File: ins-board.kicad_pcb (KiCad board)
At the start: 2 copper layers, 35 x 20 mm, 48 parts, among them P1 CONN_8, P2 PWR, U1 STM32F042C6T6, U2 MIC5201-3.3YS, U3 H3LIS331DL, U4 MPU6000, U5 LPS331AP, X1 CRYSTAL 16MHz 10ppm

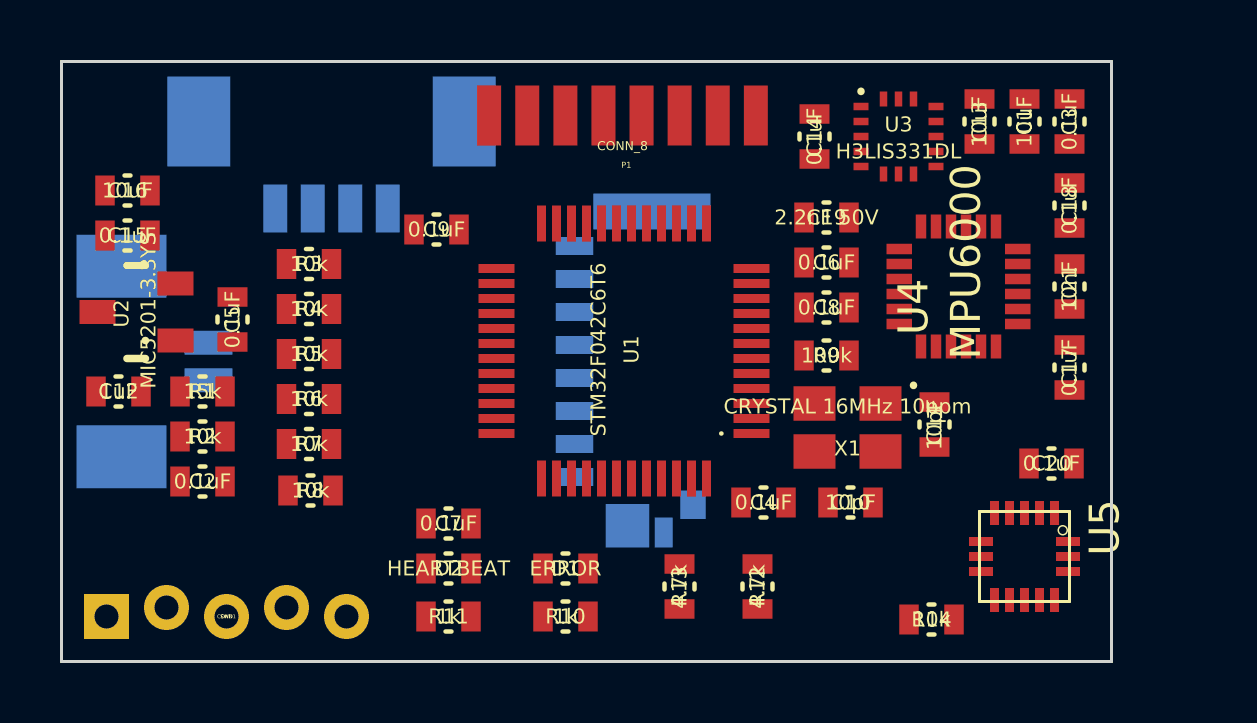
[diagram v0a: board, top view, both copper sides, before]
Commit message: Routing
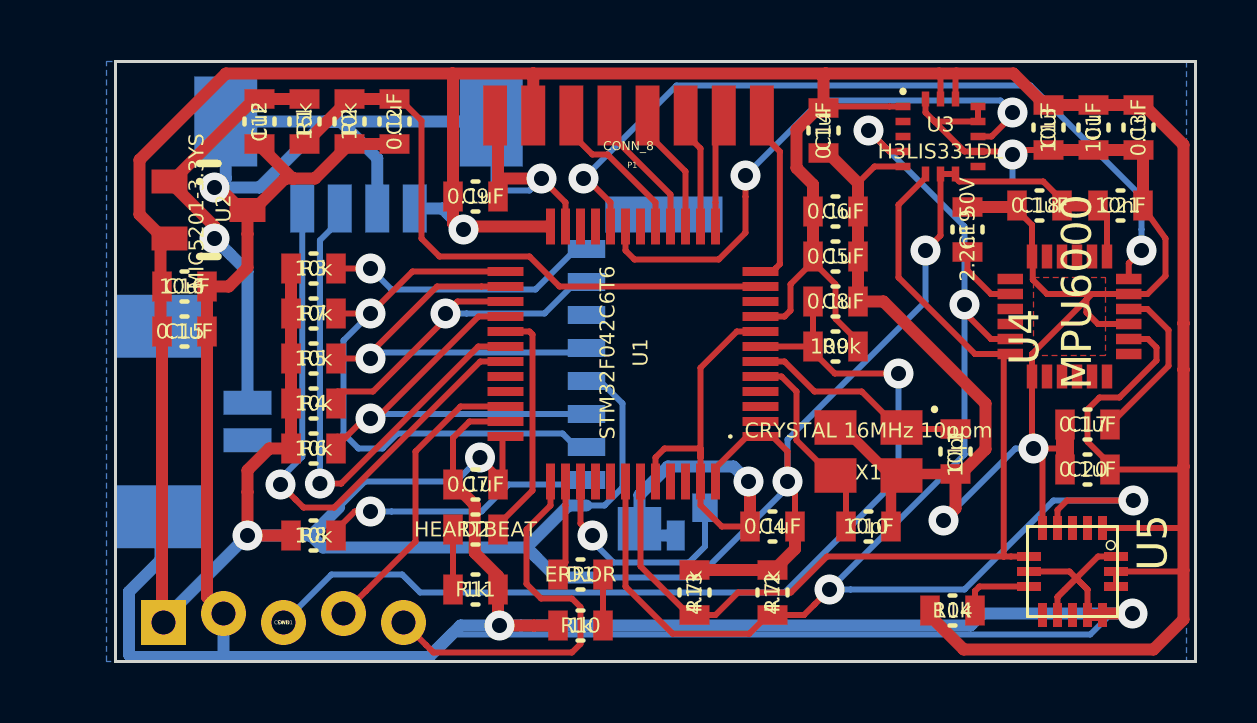
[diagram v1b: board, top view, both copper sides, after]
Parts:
- moved C5 20.2 mm to (158.8, 94.0), turned to 0 degrees
- moved C2 13.6 mm to (144.1, 89.5), turned to 270 degrees
- moved R2 11.6 mm to (142.6, 89.5), turned to 270 degrees
- moved C12 10.2 mm to (139.6, 89.5), turned to 270 degrees
- moved R1 9.62 mm to (141.1, 89.5), turned to 90 degrees
- moved U2 5.30 mm to (136.6, 91.5), turned to 270 degrees
- moved C19 4.72 mm to (163.2, 93.1), turned to 90 degrees
- moved R7 4.35 mm to (141.4, 95.9)
- moved U4 3.83 mm to (166.6, 96.0)
- moved C15 3.72 mm to (137.1, 96.5), turned to 0 degrees
- moved C16 3.72 mm to (137.1, 95.0), turned to 0 degrees
- moved C21 3.19 mm to (168.3, 92.3), turned to 0 degrees
- moved R4 3.15 mm to (141.4, 98.9)
- moved P2 2.39 mm to (136.3, 99.5)
- moved C1 2.31 mm to (167.4, 89.7)
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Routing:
- net GND: track 0.00 -> 227.3 mm, vias 0 -> 8
- net VCC: track 0.00 -> 215.9 mm, vias 0 -> 5
- net /INT_I2C_SCL: track 0.00 -> 48.3 mm, vias 0 -> 4
- net /STM32F4_NRST: track 0.00 -> 33.1 mm, vias 0 -> 1
- net /INT_I2C_SDA: track 0.00 -> 33.0 mm
- net /MPU6000_INT: track 0.00 -> 26.4 mm, vias 0 -> 2
- net /V_BAT_MON_AD: track 0.00 -> 20.7 mm
- net /UART_RX: track 0.00 -> 19.3 mm, vias 0 -> 1
- net /SD_CS: track 0.00 -> 19.3 mm, vias 0 -> 1
- net /H3LIS331DL_INT1: track 0.00 -> 18.8 mm, vias 0 -> 2
- net /UART_TX: track 0.00 -> 17.5 mm, vias 0 -> 1
- net /SD_DIN: track 0.00 -> 15.1 mm, vias 0 -> 1
- net /V_DC: track 0.00 -> 14.1 mm, vias 0 -> 1
- net /SD_CLK: track 0.00 -> 14.0 mm, vias 0 -> 1
- net /STM32F4_SWCLK: track 0.00 -> 13.5 mm
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- added copper zone on B.Cu, net GND
- added copper zone on F.Cu, net GND
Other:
- board size 35 x 20 mm -> 36 x 20 mm
- net class Default: trace_width 0.25 -> 0.2
- net class Power added: clearance 0.2, trace_width 0.3, via_dia 1, via_drill 0.5

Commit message: PCB review + corrections
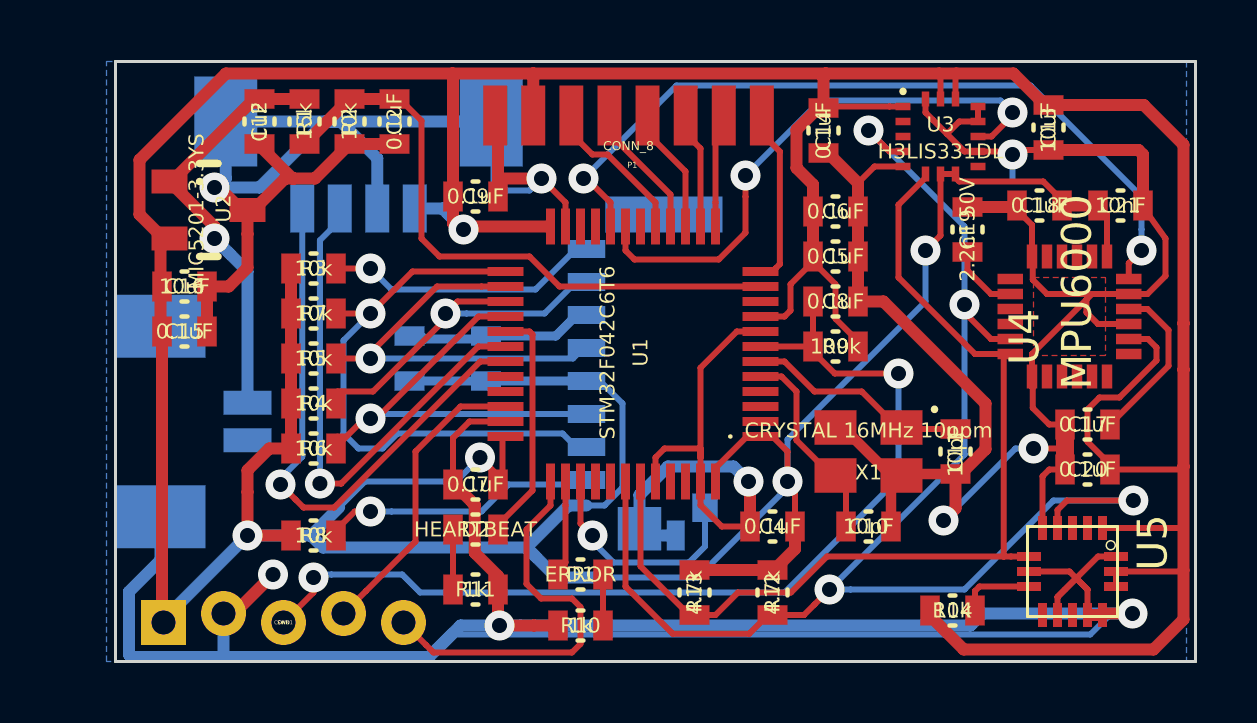
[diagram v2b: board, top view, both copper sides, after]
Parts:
- C1, C3: moved to B.Cu
- moved C1 24.1 mm to (144.6, 97.4), turned to 90 degrees
- moved C3 23.1 mm to (147.2, 97.4), turned to 90 degrees
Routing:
- net VCC: track 215.9 -> 221.8 mm
- net GND: track 227.3 -> 225.6 mm, vias 8 -> 9
- net /STM32F4_NRST: track 33.1 -> 33.4 mm, vias 1 -> 2
